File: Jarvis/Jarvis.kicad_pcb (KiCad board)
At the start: 4 copper layers, 30 x 55.1 mm, 134 parts, among them IC1 ADP1607, IC2 MAX-8Q, IC3 MPU-9250, IC4 STM32F411CxUx, IC5 Si4460, IC6 MS5611-01BA03, IC7 S25FL127S, J1 PYRO, J2 PWR, J3 ARM, J4 MICROUSB, P1 SMA, P2 SMA, P3 SWD_TC, Q1 PFET, Q2 PFET, Q3 PFET, Q4 NFET, Q5 NFET, Q6 NFET, Q7 NFET, Y1 26MHz, Y2 30MHz

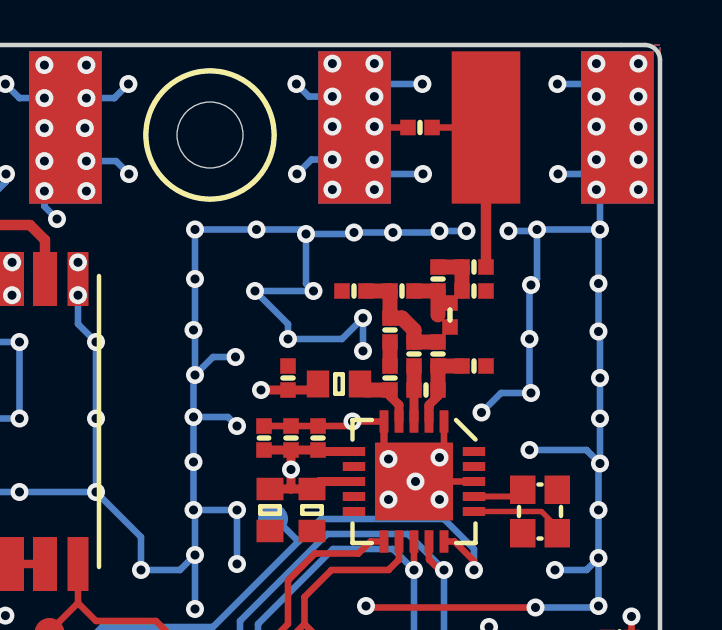
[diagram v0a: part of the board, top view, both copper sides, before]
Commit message: Tidy up before final assembly
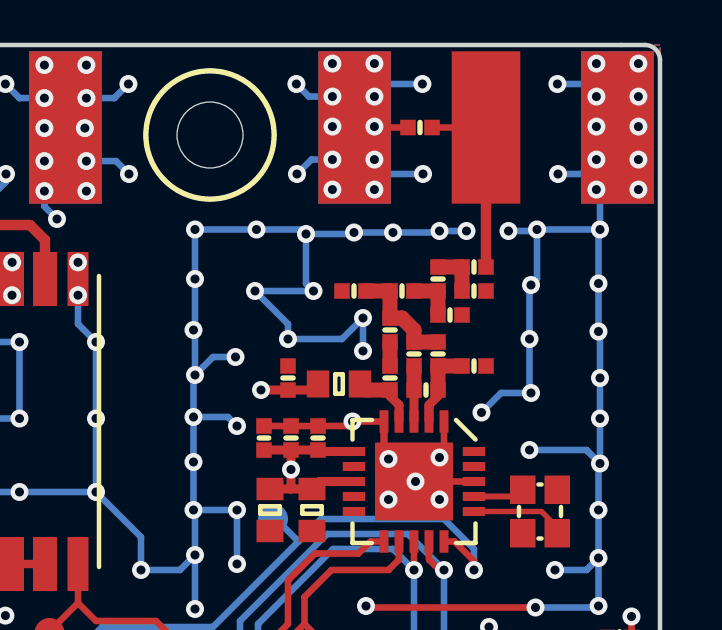
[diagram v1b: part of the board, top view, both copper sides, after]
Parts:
- turned C27 to 0 degrees
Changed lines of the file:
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@@
 (kicad_pcb (version 4) (host pcbnew 4.0.2+e4-6225~38~ubuntu14.04.1-stable)
   (general
-    (links 308)
-    (no_connects 0)
-    (area 69.827524 81.909999 129.191524 119.977524)
+    (links 342)
+    (no_connects 24)
+    (area 84.849998 74.849999 115.000001 130.100002)
     (thickness 1.6)
     (drawings 164)
@@
   )
   (module agg:0402-L (layer F.Cu)
-    (at 107.925 83.925 270)
-    (fp_text reference C27 (at -1.61 0 360) (layer F.Fab)
-      (effects (font (size 1 1) (thickness 0.15)))
-    )
-    (fp_text value 10pF (at 1.61 0 360) (layer F.Fab)
-      (effects (font (size 1 1) (thickness 0.15)))
-    )
-    (fp_line (start -0.5 -0.25) (end 0.5 -0.25) (layer F.Fab) (width 0.01))
-    (fp_line (start 0.5 -0.25) (end 0.5 0.25) (layer F.Fab) (width 0.01))
-    (fp_line (start 0.5 0.25) (end -0.5 0.25) (layer F.Fab) (width 0.01))
-    (fp_line (start -0.5 0.25) (end -0.5 -0.25) (layer F.Fab) (width 0.01))
-    (fp_line (start -0.2 -0.25) (end -0.2 0.25) (layer F.Fab) (width 0.01))
-    (fp_line (start 0.2 -0.25) (end 0.2 0.25) (layer F.Fab) (width 0.01))
-    (fp_line (start -0.8 -0.4) (end 0.8 -0.4) (layer F.CrtYd) (width 0.01))
-    (fp_line (start 0.8 -0.4) (end 0.8 0.4) (layer F.CrtYd) (width 0.01))
-    (fp_line (start 0.8 0.4) (end -0.8 0.4) (layer F.CrtYd) (width 0.01))
-    (fp_line (start -0.8 0.4) (end -0.8 -0.4) (layer F.CrtYd) (width 0.01))
-    (pad 1 smd rect (at -0.4 0 270) (size 0.52 0.52) (layers F.Cu F.Paste F.Mask)
+    (at 107.925 83.925)
+    (fp_text reference C27 (at -1.61 0 90) (layer F.Fab)
+      (effects (font (size 1 1) (thickness 0.15)))
+    )
+    (fp_text value 10pF (at 1.61 0 90) (layer F.Fab)
+      (effects (font (size 1 1) (thickness 0.15)))
+    )
+    (fp_line (start -0.5 -0.25) (end 0.5 -0.25) (layer F.Fab) (width 0.01))
+    (fp_line (start 0.5 -0.25) (end 0.5 0.25) (layer F.Fab) (width 0.01))
+    (fp_line (start 0.5 0.25) (end -0.5 0.25) (layer F.Fab) (width 0.01))
+    (fp_line (start -0.5 0.25) (end -0.5 -0.25) (layer F.Fab) (width 0.01))
+    (fp_line (start -0.2 -0.25) (end -0.2 0.25) (layer F.Fab) (width 0.01))
+    (fp_line (start 0.2 -0.25) (end 0.2 0.25) (layer F.Fab) (width 0.01))
+    (fp_line (start -0.8 -0.4) (end 0.8 -0.4) (layer F.CrtYd) (width 0.01))
+    (fp_line (start 0.8 -0.4) (end 0.8 0.4) (layer F.CrtYd) (width 0.01))
+    (fp_line (start 0.8 0.4) (end -0.8 0.4) (layer F.CrtYd) (width 0.01))
+    (fp_line (start -0.8 0.4) (end -0.8 -0.4) (layer F.CrtYd) (width 0.01))
+    (pad 1 smd rect (at -0.4 0) (size 0.52 0.52) (layers F.Cu F.Paste F.Mask)
       (net 44 "Net-(C27-Pad1)"))
-    (pad 2 smd rect (at 0.4 0 270) (size 0.52 0.52) (layers F.Cu F.Paste F.Mask)
-      (net 2 GND))
-  )
+    (pad 2 smd rect (at 0.4 0) (size 0.52 0.52) (layers F.Cu F.Paste F.Mask)
+      (net 2 GND))
+  )
